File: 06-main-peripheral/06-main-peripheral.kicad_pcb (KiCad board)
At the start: 4 copper layers, 58.5 x 29.2 mm, 17 parts, among them J1 T4040014041000, J2 FH-41-15S-0.5SH-05_, J3 T4040014041000, J4 T4040014041000, Q1 DMN3018SSD-13, SW1 100SP1K1B25M1QEH-ND, U1 LM74700-Q1

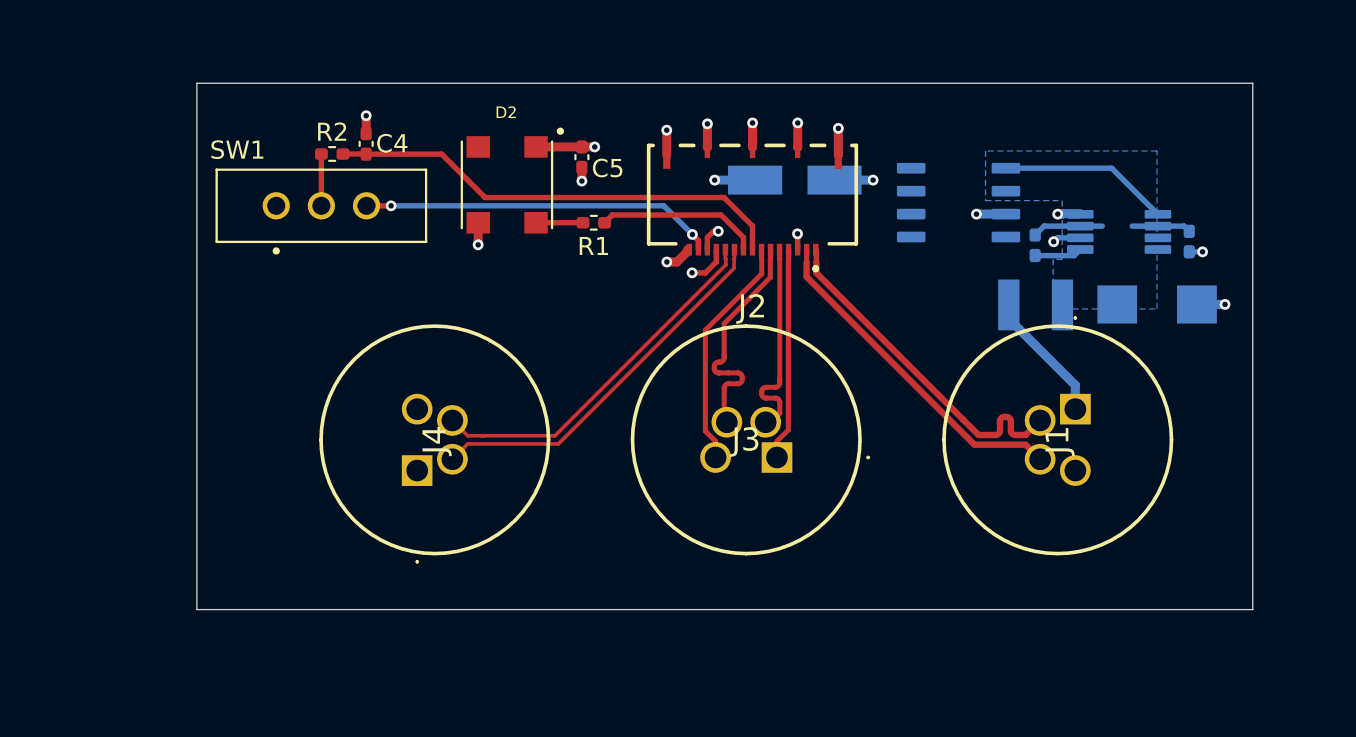
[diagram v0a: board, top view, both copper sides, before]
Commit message: before revision from overlords
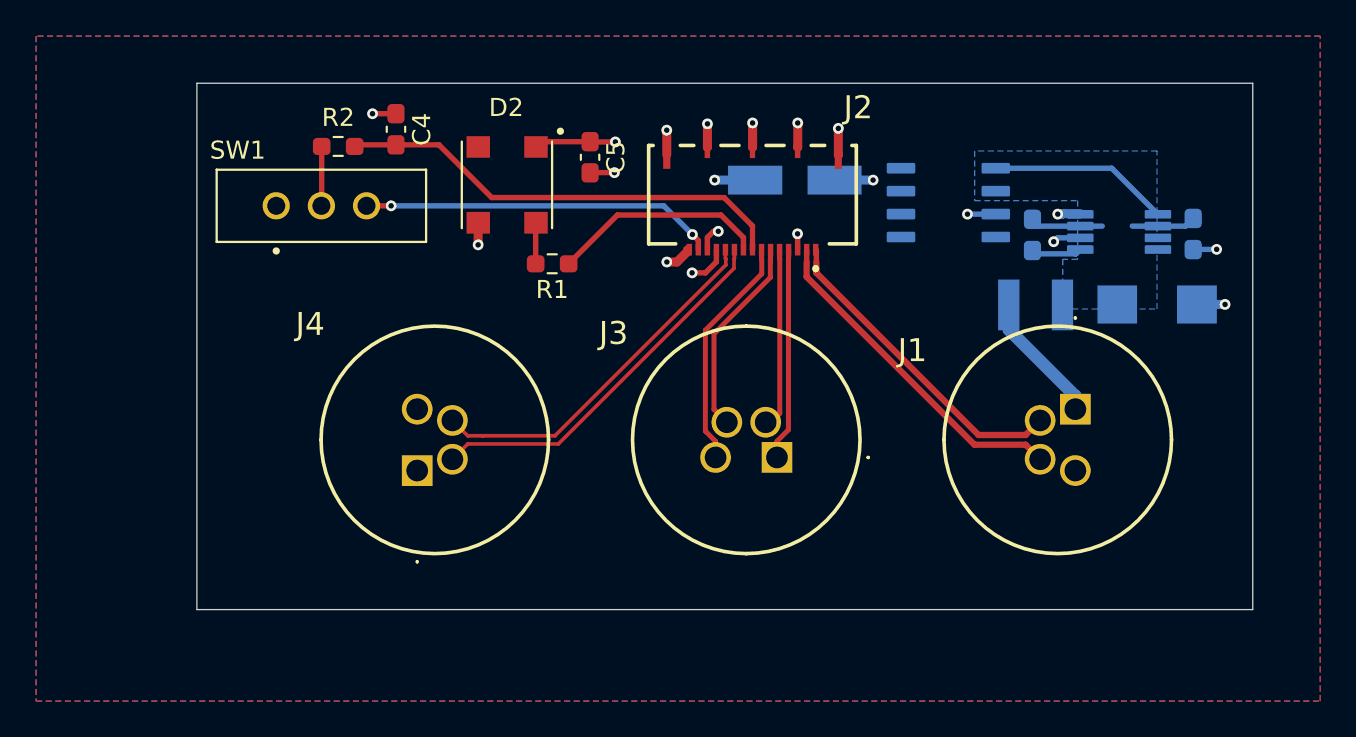
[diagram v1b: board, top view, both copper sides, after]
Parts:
- C1, C3, C4, C5: footprint Capacitor_SMD:C_0402_1005Metric_Pad0.74x0.62mm_HandSolder -> Capacitor_SMD:C_0603_1608Metric_Pad1.08x0.95mm_HandSolder
- R1, R2: footprint Resistor_SMD:R_0402_1005Metric_Pad0.72x0.64mm_HandSolder -> Resistor_SMD:R_0603_1608Metric_Pad0.98x0.95mm_HandSolder
- moved R1 3.24 mm to (150.5, 85.0)
- moved C4 1.84 mm to (141.8, 77.5)
- moved C3 0.59 mm to (177.1, 83.4)
- moved Q1 0.56 mm to (172.4, 81.6)
- moved R2 0.53 mm to (138.7, 78.5)
- moved C1 0.47 mm to (186.0, 83.3)
- moved C5 0.45 mm to (152.6, 79.1)
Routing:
- net LED_CONTROL: track 9.06 -> 12.0 mm
- net TX_N: track 13.1 -> 11.1 mm
- net USB_D_N: track 19.3 -> 17.7 mm
- net RX_N: track 11.6 -> 10.1 mm
- net GND: track 18.9 -> 20.4 mm
- net 5V: track 4.74 -> 6.01 mm
- added copper zone on B.Cu, net GND
- added copper zone on F.Cu, net GND
